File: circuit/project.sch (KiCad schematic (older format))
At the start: 8 parts

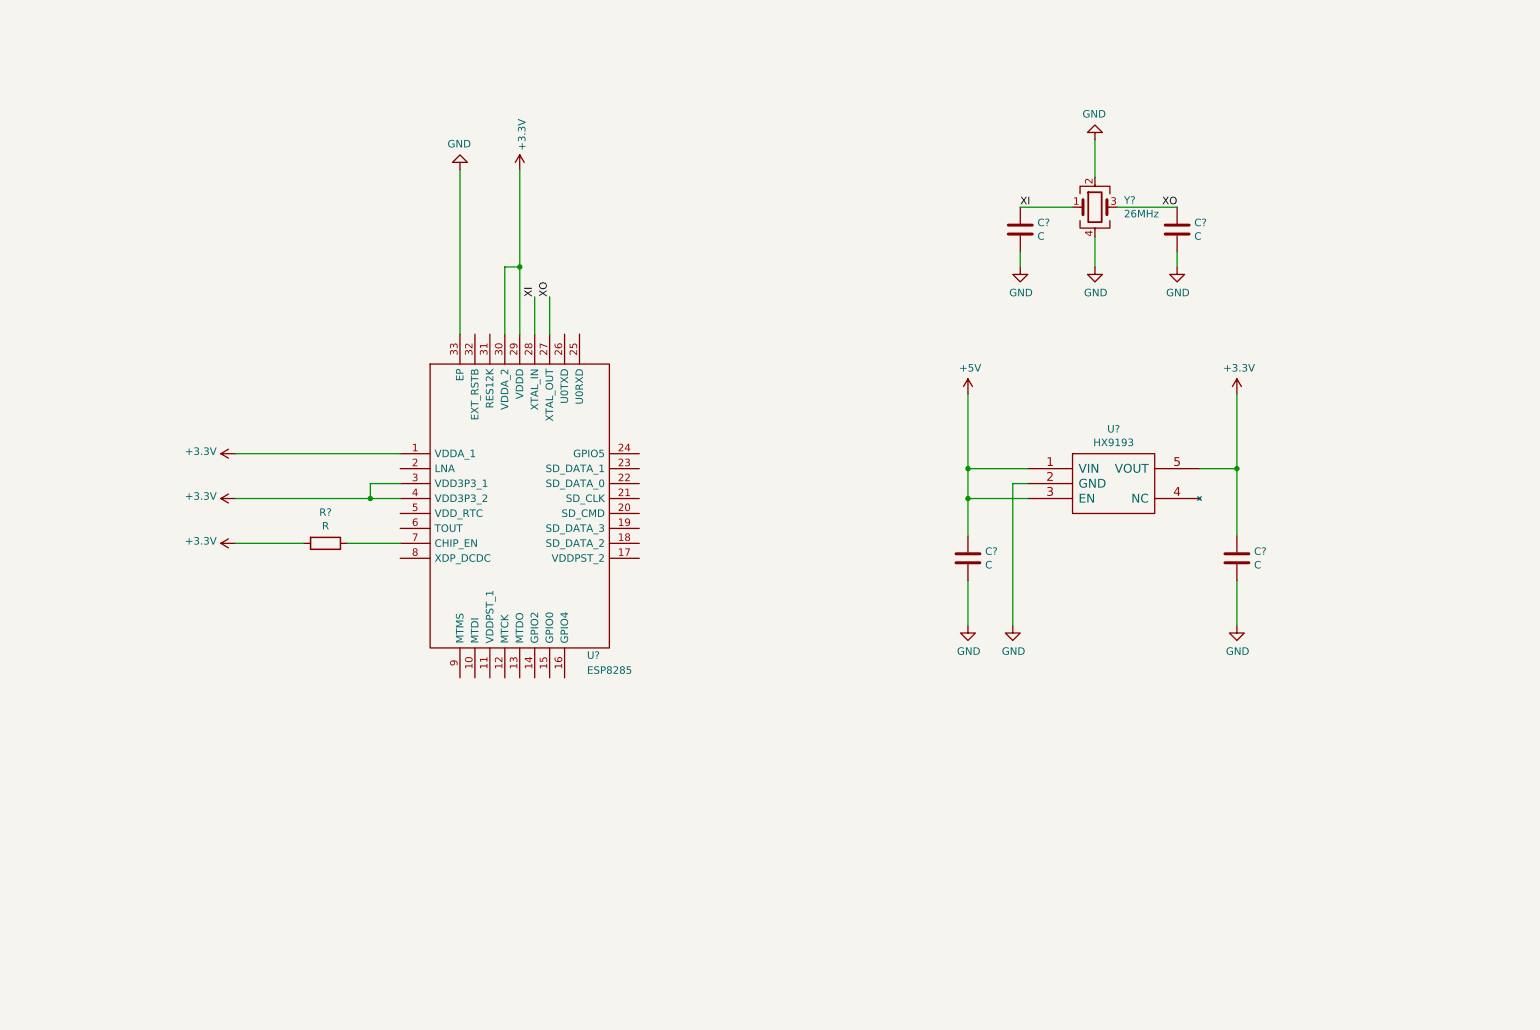
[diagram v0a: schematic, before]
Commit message: Finished circuit design
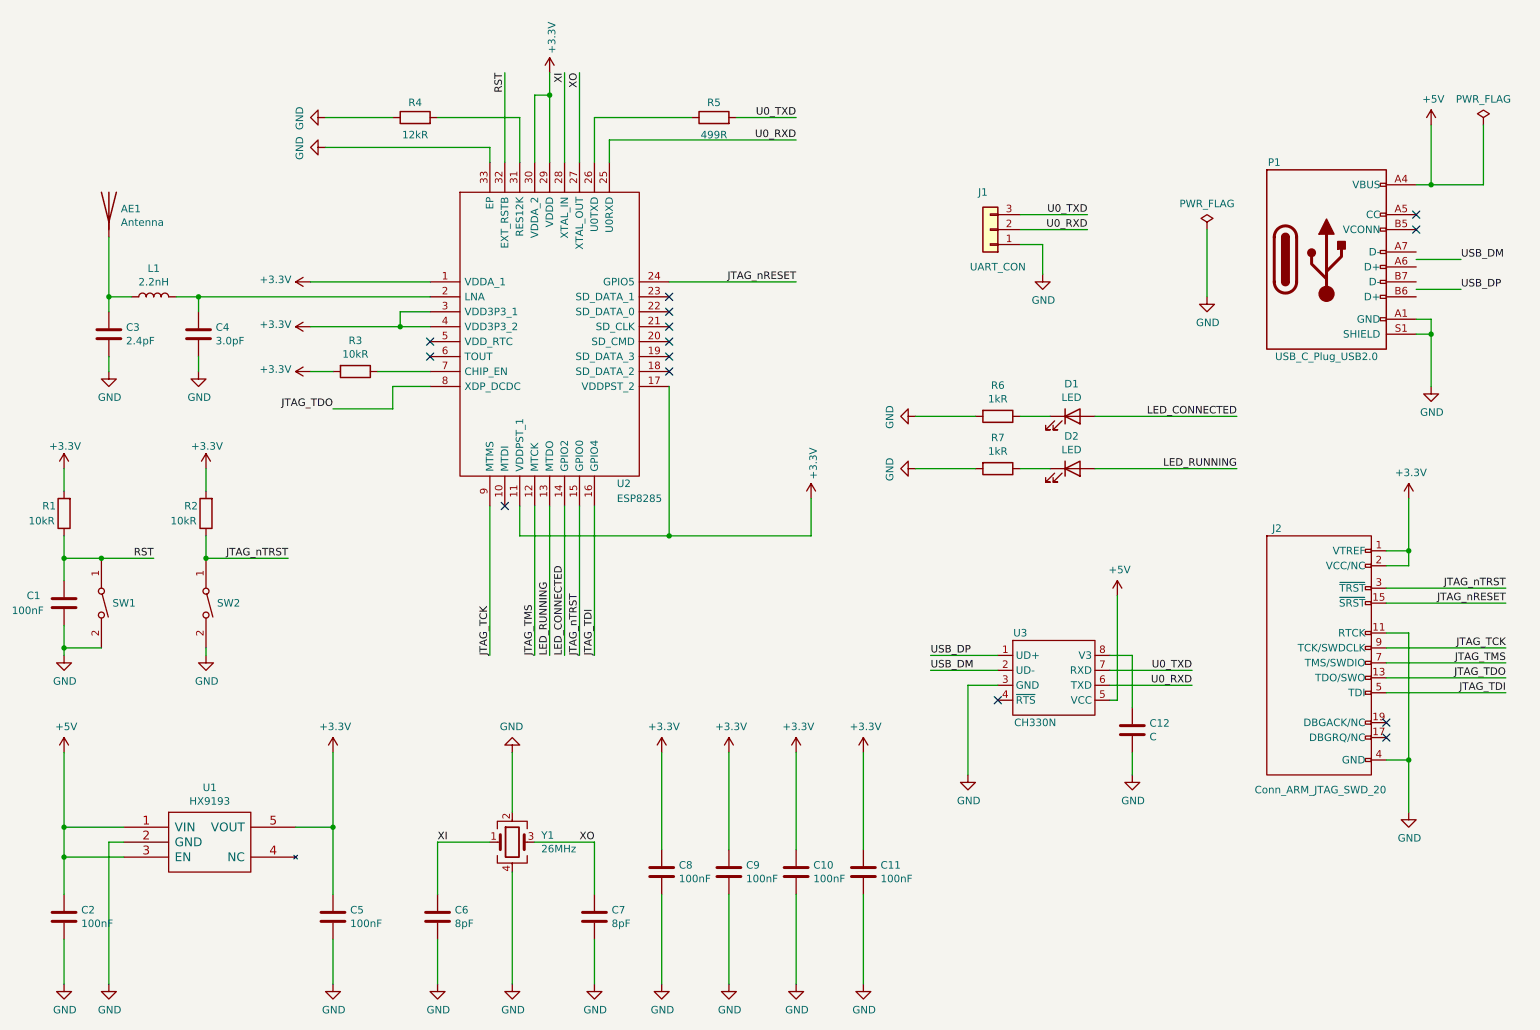
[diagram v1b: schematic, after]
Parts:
- added AE1: Antenna, symbol Device:Antenna
- added C1, C10, C11, C8, C9: 100nF, symbol Device:C
- added C12: C, symbol Device:C
- added C3: 2.4pF, symbol Device:C
- added C4: 3.0pF, symbol Device:C
- added D1, D2: LED, symbol Device:LED
- added J1: UART_CON, symbol Connector_Generic:Conn_01x03
- added J2: Conn_ARM_JTAG_SWD_20, symbol Connector:Conn_ARM_JTAG_SWD_20
- added L1: 2.2nH, symbol Device:L
- added P1: USB_C_Plug_USB2.0, symbol Connector:USB_C_Plug_USB2.0
- added R1, R2: 10kR, symbol Device:R
- added R4: 12kR, symbol Device:R
- added R5: 499R, symbol Device:R
- added R6, R7: 1kR, symbol Device:R
- added SW1, SW2: SW_DIP_x01, symbol Switch:SW_DIP_x01
- added U3: CH330N, Package_SO:SOIC-8_3.9x4.9mm_P1.27mm, symbol Interface_USB:CH330N
- C2, C5: renamed from C?; value C -> 100nF
- C6, C7: renamed from C?; value C -> 8pF
- R3: renamed from R?; value R -> 10kR
- gave numbers to parts that had none: 3
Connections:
- net +3V3: now also U2.11 (VDDPST_1), U2.17 (VDDPST_2), C10.1, C11.1, C8.1, C9.1, J2.1 (VTREF), J2.2 (VCC/NC), R1.2, R2.2
- net +5V: now also P1.A4 (VBUS), P1.A9 (VBUS), P1.B4 (VBUS), P1.B9 (VBUS), U3.5 (VCC)
- net GND: now also C1.2, C10.2, C11.2, C12.2, C3.2, C4.2, C8.2, C9.2, J1.1 (Pin_1), J2.10 (GND), J2.11 (RTCK), J2.12 (GND), J2.14 (GND), J2.16 (GND), J2.18 (GND), J2.20 (GND), J2.4 (GND), J2.6 (GND), J2.8 (GND), P1.A1 (GND), P1.A12 (GND), P1.B1 (GND), P1.B12 (GND), P1.S1 (SHIELD), R4.1, R6.2, R7.2, SW1.2, SW2.2, U3.3 (GND)
- net JTAG_TMS: now reaches U2.12 (MTCK)
- net JTAG_TMS: now also J2.7 (TMS/SWDIO)
- net LED_RUNNING: now reaches U2.13 (MTDO)
- net LED_RUNNING: now also D2.2 (A)
- net LED_CONNECTED: now reaches U2.14 (GPIO2)
- net LED_CONNECTED: now also D1.2 (A)
- net JTAG_nTRST: now reaches U2.15 (GPIO0)
- net JTAG_nTRST: now also J2.3 (~TRST~), R2.1, SW2.1
- net JTAG_TDI: now reaches U2.16 (GPIO4)
- net JTAG_TDI: now also J2.5 (TDI)
- net at U2.2 (LNA): now also C4.1, L1.2
- net JTAG_nRESET: now reaches U2.24 (GPIO5)
- net JTAG_nRESET: now also J2.15 (~SRST~)
- net U0_RXD: now reaches U2.25 (U0RXD)
- net U0_RXD: now also J1.2 (Pin_2), U3.6 (TXD)
- net at U2.26 (U0TXD): now also R5.1
- net at U2.31 (RES12K): now also R4.2
- net RST: now reaches U2.32 (EXT_RSTB)
- net RST: now also C1.1, R1.1, SW1.1
- net JTAG_TDO: now reaches U2.8 (XDP_DCDC)
- net JTAG_TDO: now also J2.13 (TDO/SWO)
- net JTAG_TCK: now reaches U2.9 (MTMS)
- net JTAG_TCK: now also J2.9 (TCK/SWDCLK)
- new net: AE1.1 (A), C3.1, L1.1
- new net: C12.1, U3.8 (V3)
- new net: D2.1 (K), R7.1
- new net: D1.1 (K), R6.1
- new net U0_TXD: J1.3 (Pin_3), R5.2, U3.7 (RXD)
- new net USB_DM: U3.2 (UD-)
- new net USB_DP: U3.1 (UD+)
- no-connect marks 0 -> 14
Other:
- moved on the sheet: C2, C5, C6, C7, R3, U1, U2, Y1

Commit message: finished PCB design
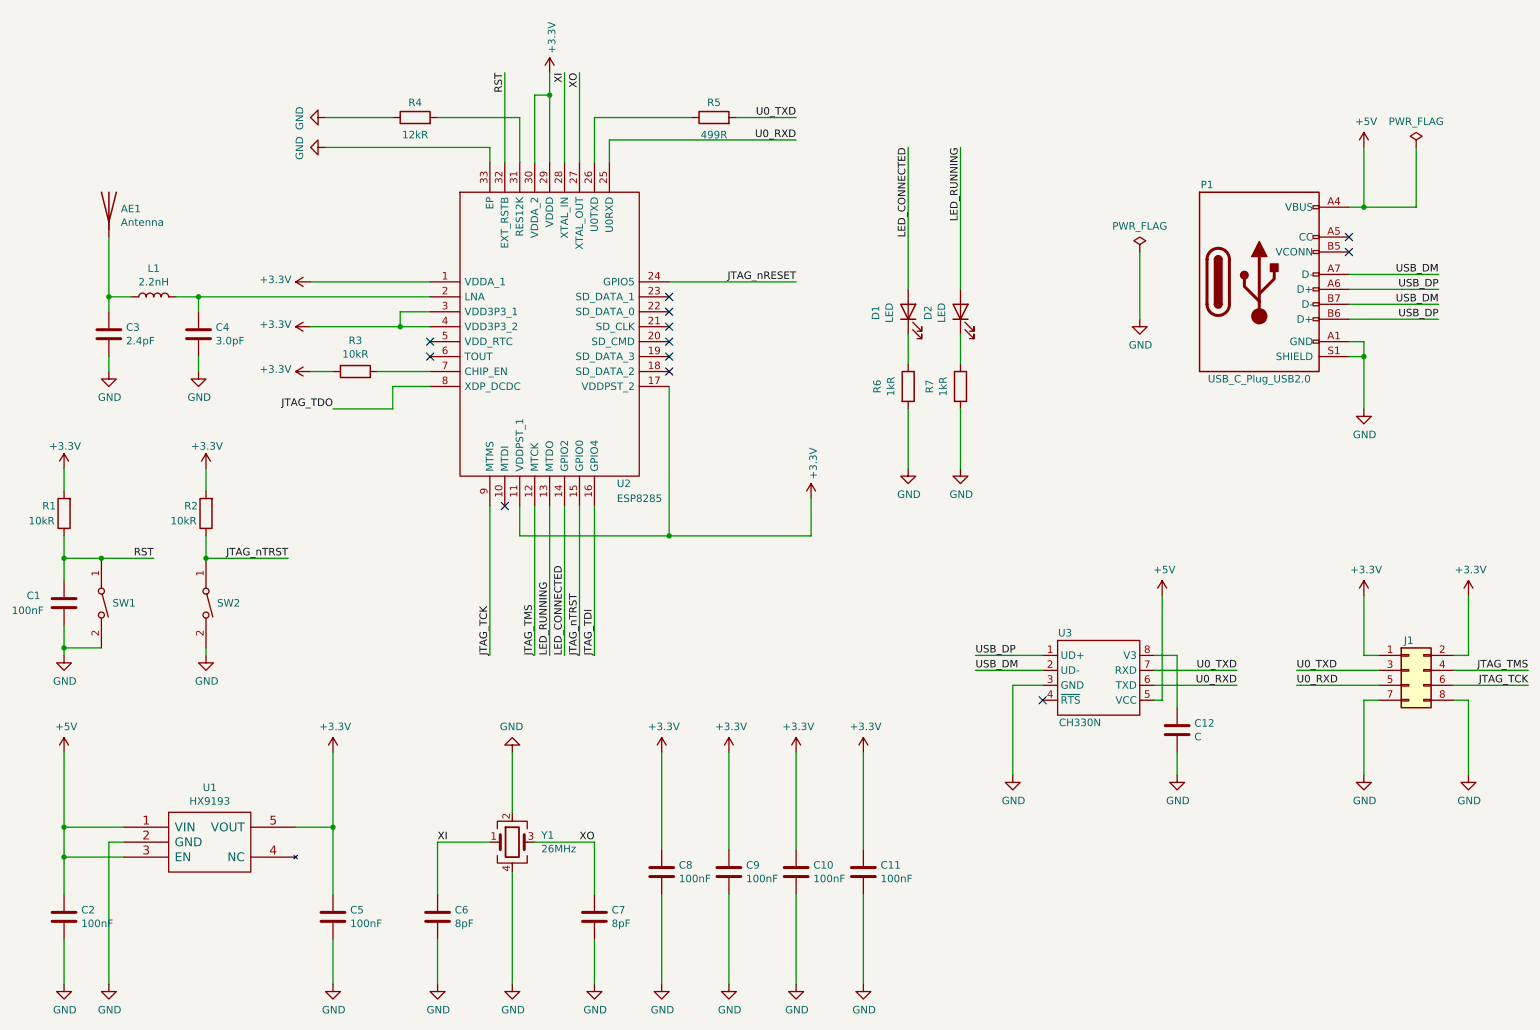
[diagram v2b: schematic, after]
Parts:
- removed J1: UART_CON, symbol Connector_Generic:Conn_01x03
- removed J2: Conn_ARM_JTAG_SWD_20, symbol Connector:Conn_ARM_JTAG_SWD_20
- added J1: Conn_02x04_Odd_Even, Connector_PinHeader_1.27mm:PinHeader_2x04_P1.27mm_Vertical_SMD, symbol Connector_Generic:Conn_02x04_Odd_Even
- AE1: footprint (none) -> RF_Antenna:Johanson_2450AT18x100
- C1, C10, C11, C12, C2, C3, C4, C5, C6, C7, C8, C9: footprint (none) -> Capacitor_SMD:C_0603_1608Metric
- D1, D2: footprint (none) -> LED_SMD:LED_0603_1608Metric_Castellated
- L1: footprint (none) -> Inductor_SMD:L_0603_1608Metric
- P1: footprint (none) -> Connector_USB:USB_C_Receptacle_HRO_TYPE-C-31-M-12
- R1, R2, R3, R4, R5, R6, R7: footprint (none) -> Resistor_SMD:R_0603_1608Metric
- SW1, SW2: footprint (none) -> Button_Switch_SMD:SW_Push_SPST_NO_Alps_SKRK
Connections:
- net +3V3: now also J1.1 (Pin_1), J1.2 (Pin_2)
- net GND: now also J1.7 (Pin_7), J1.8 (Pin_8)
- net JTAG_TCK: now also J1.6 (Pin_6)
- net JTAG_TMS: now also J1.4 (Pin_4)
- net U0_RXD: now also J1.5 (Pin_5)
- net U0_TXD: now also J1.3 (Pin_3)
- net USB_DM: now also P1.A7 (D-), P1.B7 (D-)
- net USB_DP: now also P1.A6 (D+), P1.B6 (D+)
- no-connect marks 14 -> 12
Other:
- moved on the sheet: C12, D1, D2, P1, R6, R7, U3
